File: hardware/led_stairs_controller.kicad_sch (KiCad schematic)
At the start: 151 parts, among them J1 DIN41612_02x32_AC, J11 DIN41612_02x32_AC, J19 Conn_01x05_Pin, Q1 IRF7341PBF, Q10 IRF7341PBF, Q11 IRF7341PBF, Q12 IRF7341PBF, Q13 IRF7341PBF, Q14 IRF7341PBF, Q15 IRF7341PBF, Q16 IRF7341PBF, Q17 BSS138, Q18 BSS138, Q19 BSS138, Q2 IRF7341PBF, Q20 BSS138, Q3 IRF7341PBF, Q4 IRF7341PBF, Q5 IRF7341PBF, Q6 IRF7341PBF, Q7 IRF7341PBF, Q8 IRF7341PBF, Q9 IRF7341PBF, U1 PCA9635, U10 PCA9635, U2 ESP32-DEVKITC-32UE, U3 PC817, U4 MCP23008-xSO, U5 PC817, U6 PC817, U7 PC817, U8 R-78E5.0-1.0, U9 CD74HC4067M

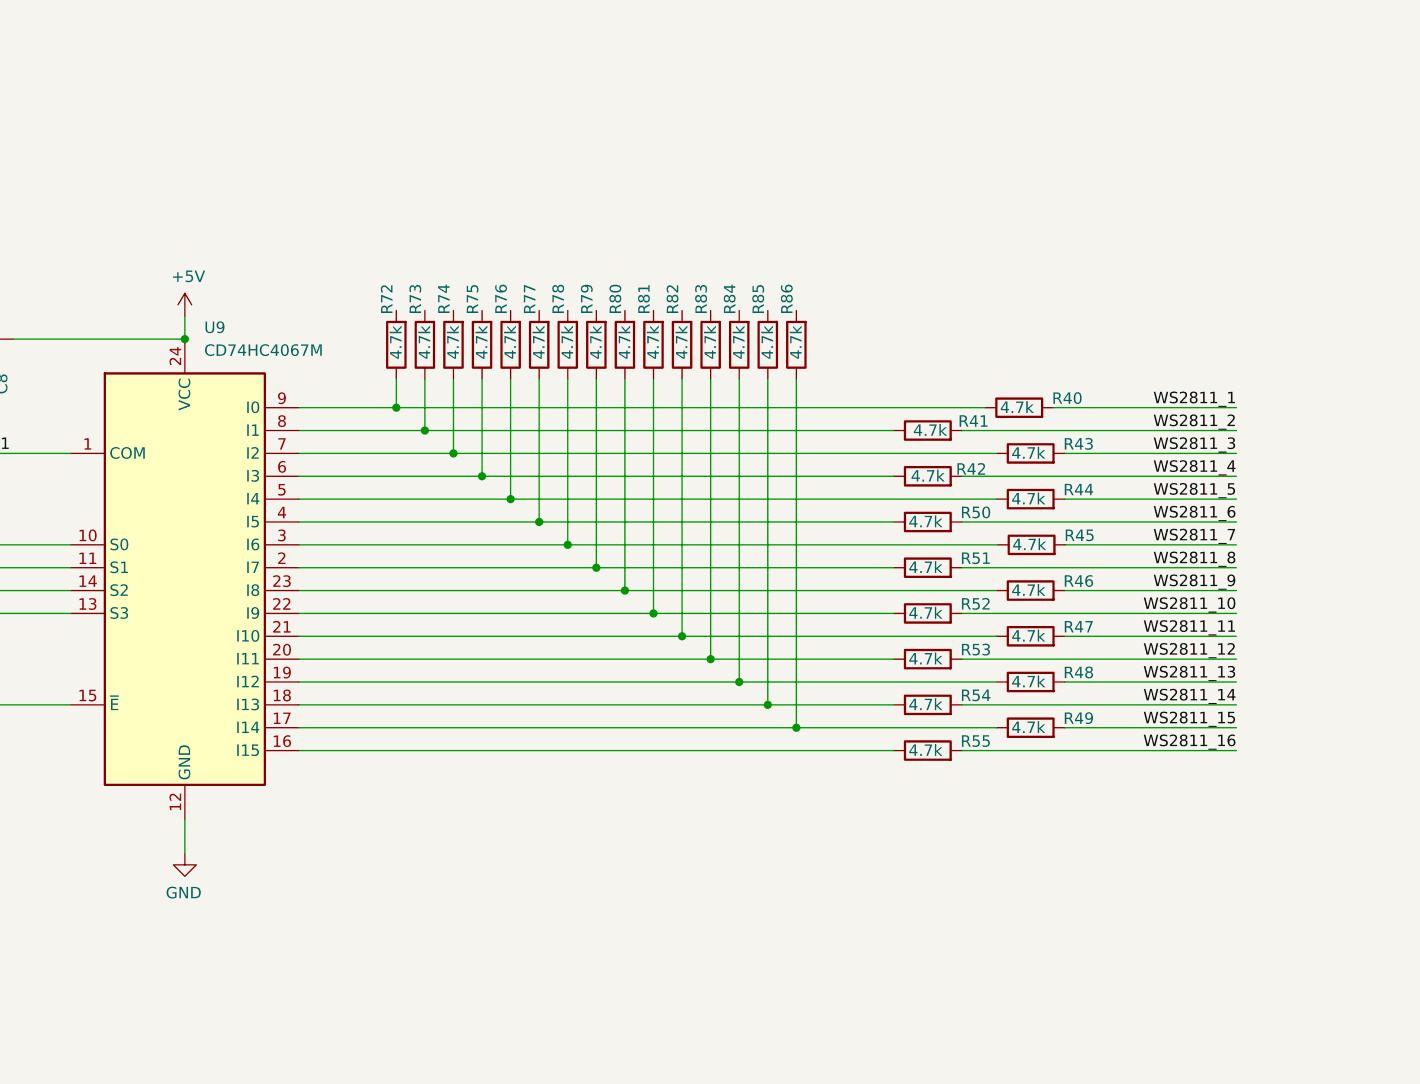
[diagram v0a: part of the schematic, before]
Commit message: update
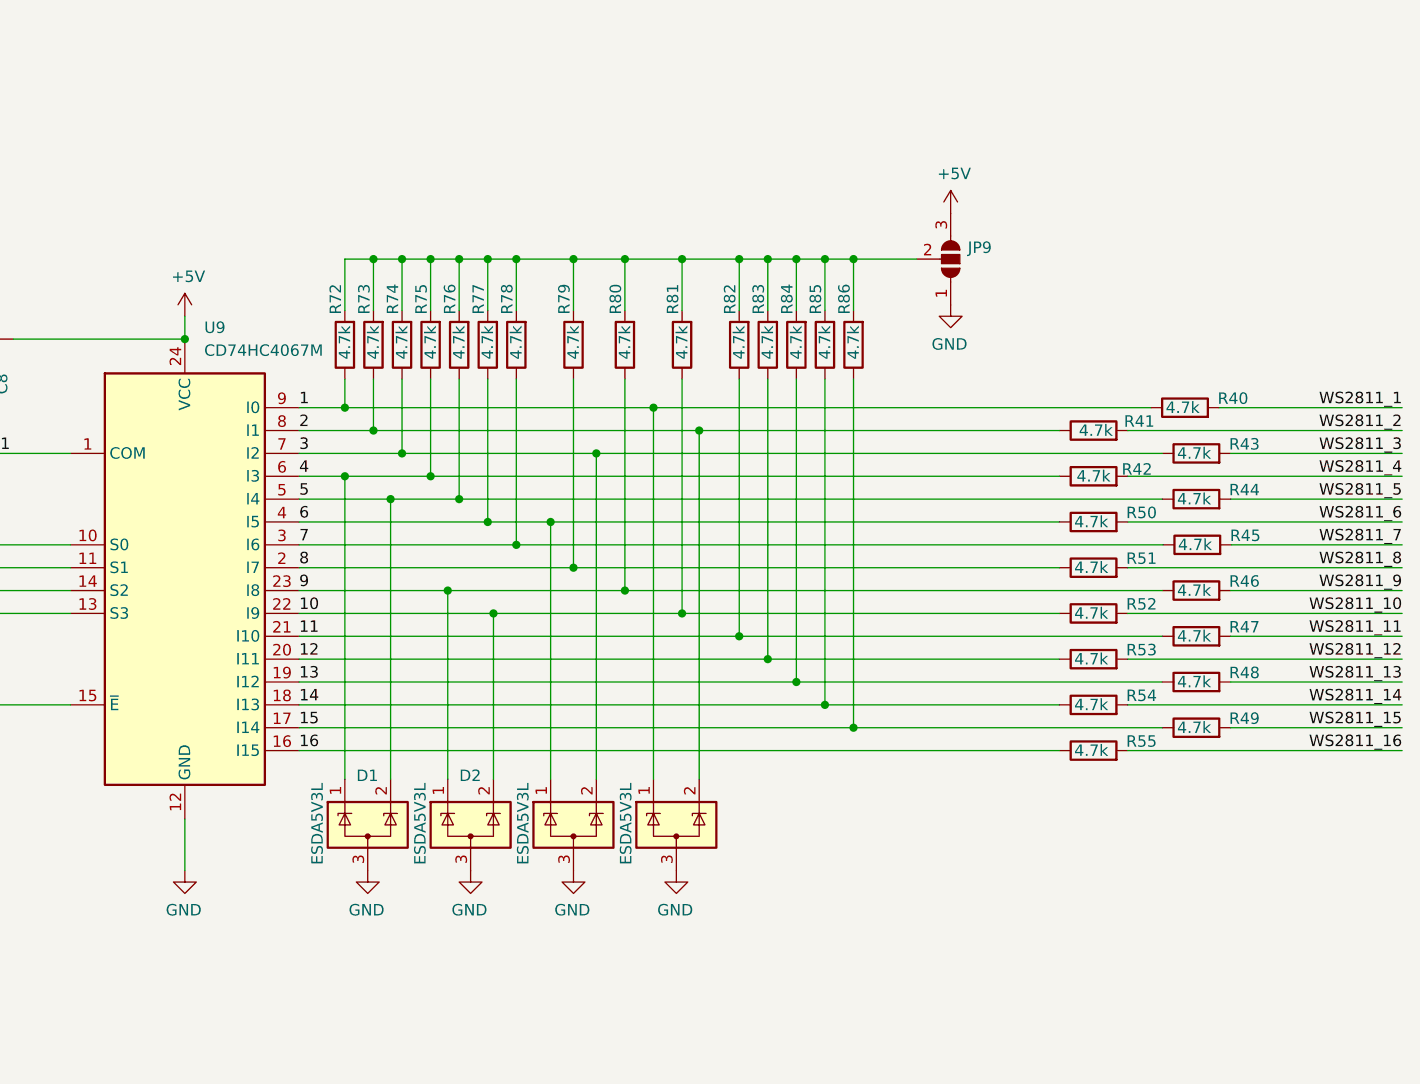
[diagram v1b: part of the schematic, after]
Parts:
- added D1, D2, D3, D4: ESDA5V3L, Package_TO_SOT_SMD:SOT-23-3, symbol Power_Protection:ESDA5V3L
- added JP9: SolderJumper_3_Open, Jumper:SolderJumper-3_P1.3mm_Open_RoundedPad1.0x1.5mm_NumberLabels, symbol Jumper:SolderJumper_3_Open
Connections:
- net +5V: now also JP9.3 (B)
- net GND: now also D1.3 (A), D2.3 (A), D3.3 (A), D4.3 (A), JP9.1 (A)
- net 4: now reaches R42.1, R75.1, U9.6 (I3)
- net 4: now also D1.1 (K)
- net 7: now reaches R45.1, R78.1, U9.3 (I6)
- net at R78.2: now also R72.2, R73.2, R74.2, R75.2, R76.2, R77.2, R79.2, R80.2, R81.2, R82.2, R83.2, R84.2, R85.2, R86.2, JP9.2 (C)
- net 12: now reaches R53.1, R83.1, U9.20 (I11)
- net 1: now reaches R40.1, R72.1, U9.9 (I0)
- net 1: now also D4.1 (K)
- net 10: now reaches R52.1, R81.1, U9.22 (I9)
- net 10: now also D2.2 (K)
- net 15: now reaches R49.1, R86.1, U9.17 (I14)
- net 9: now reaches R46.1, R80.1, U9.23 (I8)
- net 9: now also D2.1 (K)
- net 5: now reaches R44.1, R76.1, U9.5 (I4)
- net 5: now also D1.2 (K)
- net 13: now reaches R48.1, R84.1, U9.19 (I12)
- net 3: now reaches R43.1, R74.1, U9.7 (I2)
- net 3: now also D3.2 (K)
- net 8: now reaches R51.1, R79.1, U9.2 (I7)
- net 16: now reaches R55.1, U9.16 (I15)
- net 6: now reaches R50.1, R77.1, U9.4 (I5)
- net 6: now also D3.1 (K)
- net 2: now reaches R41.1, R73.1, U9.8 (I1)
- net 2: now also D4.2 (K)
- net 14: now reaches R54.1, R85.1, U9.18 (I13)
- net 11: now reaches R47.1, R82.1, U9.21 (I10)
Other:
- moved on the sheet: R40, R41, R42, R43, R44, R45, R46, R47, R48, R49, R50, R51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

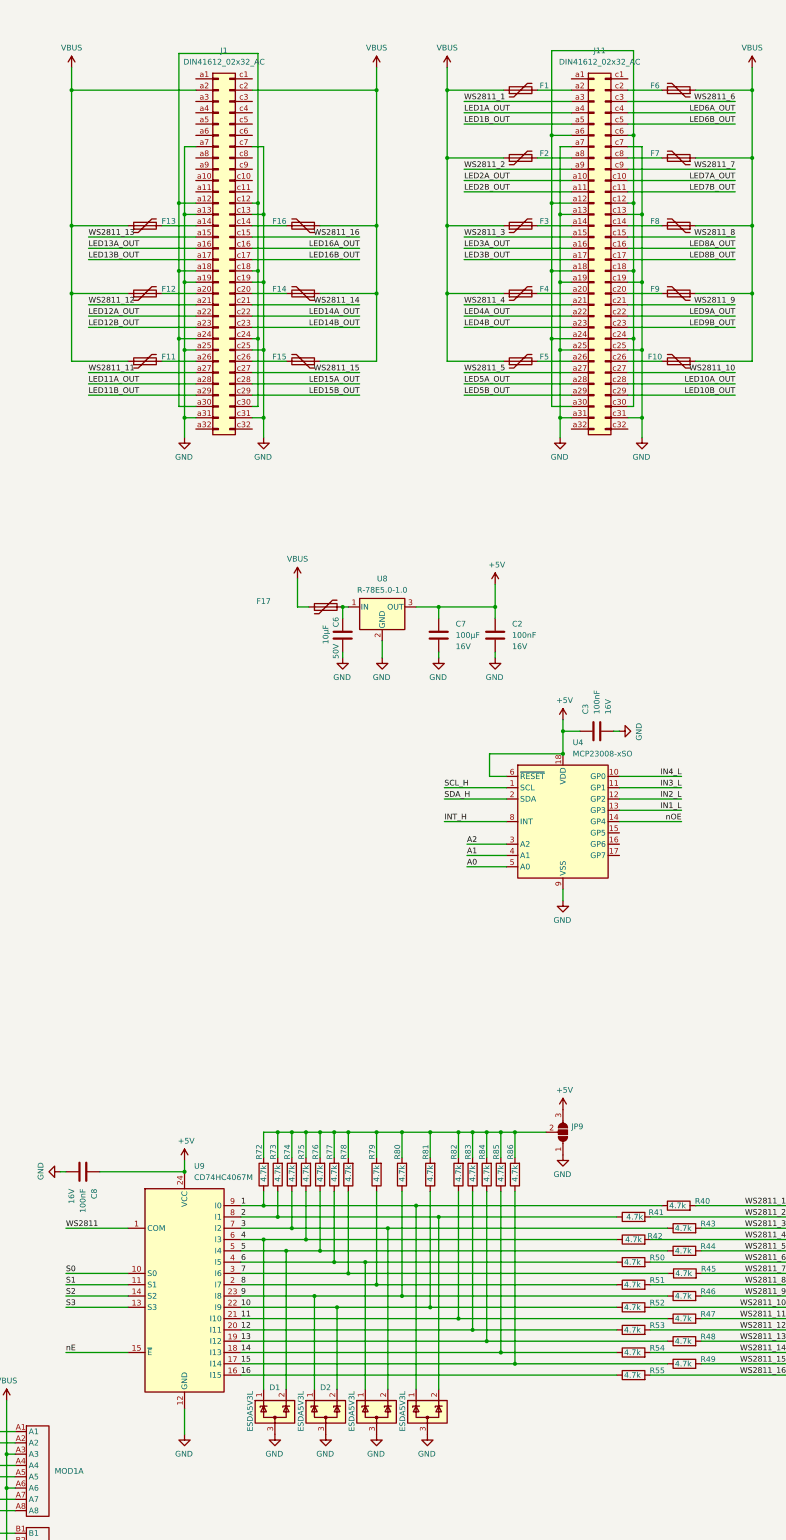
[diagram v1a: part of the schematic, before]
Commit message: update
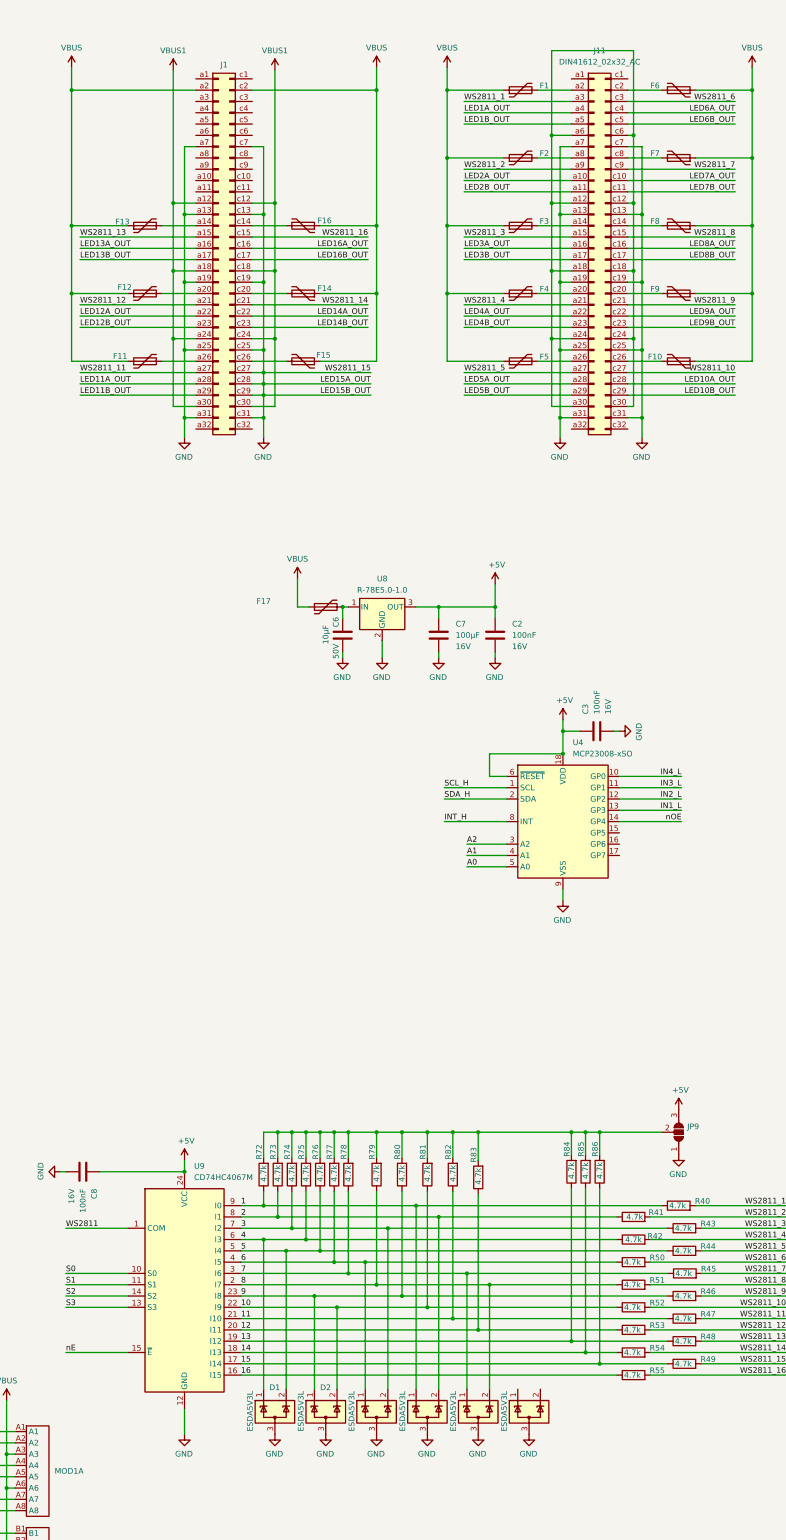
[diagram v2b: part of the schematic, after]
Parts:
- added D5, D6: ESDA5V3L, Package_TO_SOT_SMD:SOT-23-3, symbol Power_Protection:ESDA5V3L
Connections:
- net LED15A_OUT is gone; now on net GND: J1.c28 (Pin_c28), Q15.7 (D1), Q15.8 (D1)
- net LED15B_OUT is gone; now on net GND: J1.c29 (Pin_c29), Q15.5 (D2), Q15.6 (D2)
- net WS2811_15 is gone; now on net GND: J1.c27 (Pin_c27), R49.2
- net 7: now also D5.1 (K)
- net 8: now also D5.2 (K)
- net GND: now also D5.3 (A), D6.3 (A)
- net VBUS1: now reaches J1.a12 (Pin_a12), J1.a18 (Pin_a18), J1.a24 (Pin_a24), J1.a30 (Pin_a30), J1.c12 (Pin_c12), J1.c18 (Pin_c18), J1.c24 (Pin_c24), J1.c30 (Pin_c30)
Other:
- moved on the sheet: JP9, R81, R82, R83, R84, R85, R86
